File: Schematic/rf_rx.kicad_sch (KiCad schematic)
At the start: 12 parts, among them SW2 TS24CA, U1 ME6217C33M5G, U12 ESP-01F-2M, U13 E28-2G4M27SX

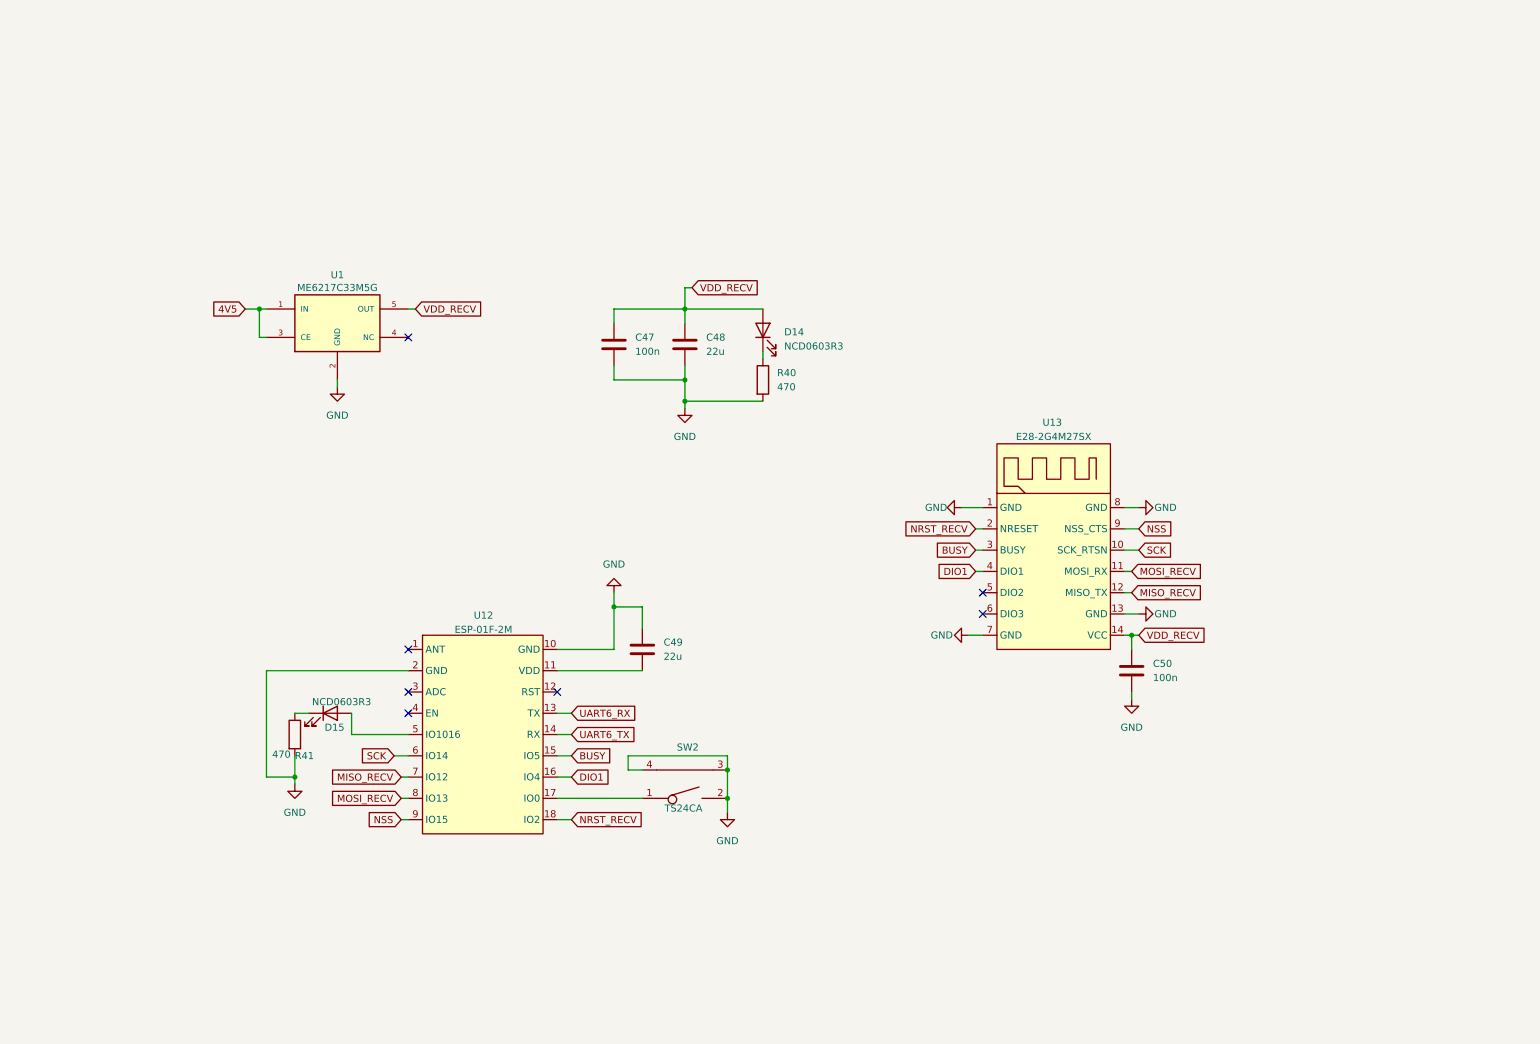
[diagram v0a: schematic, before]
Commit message: Refactor code structure for improved readability and maintainability
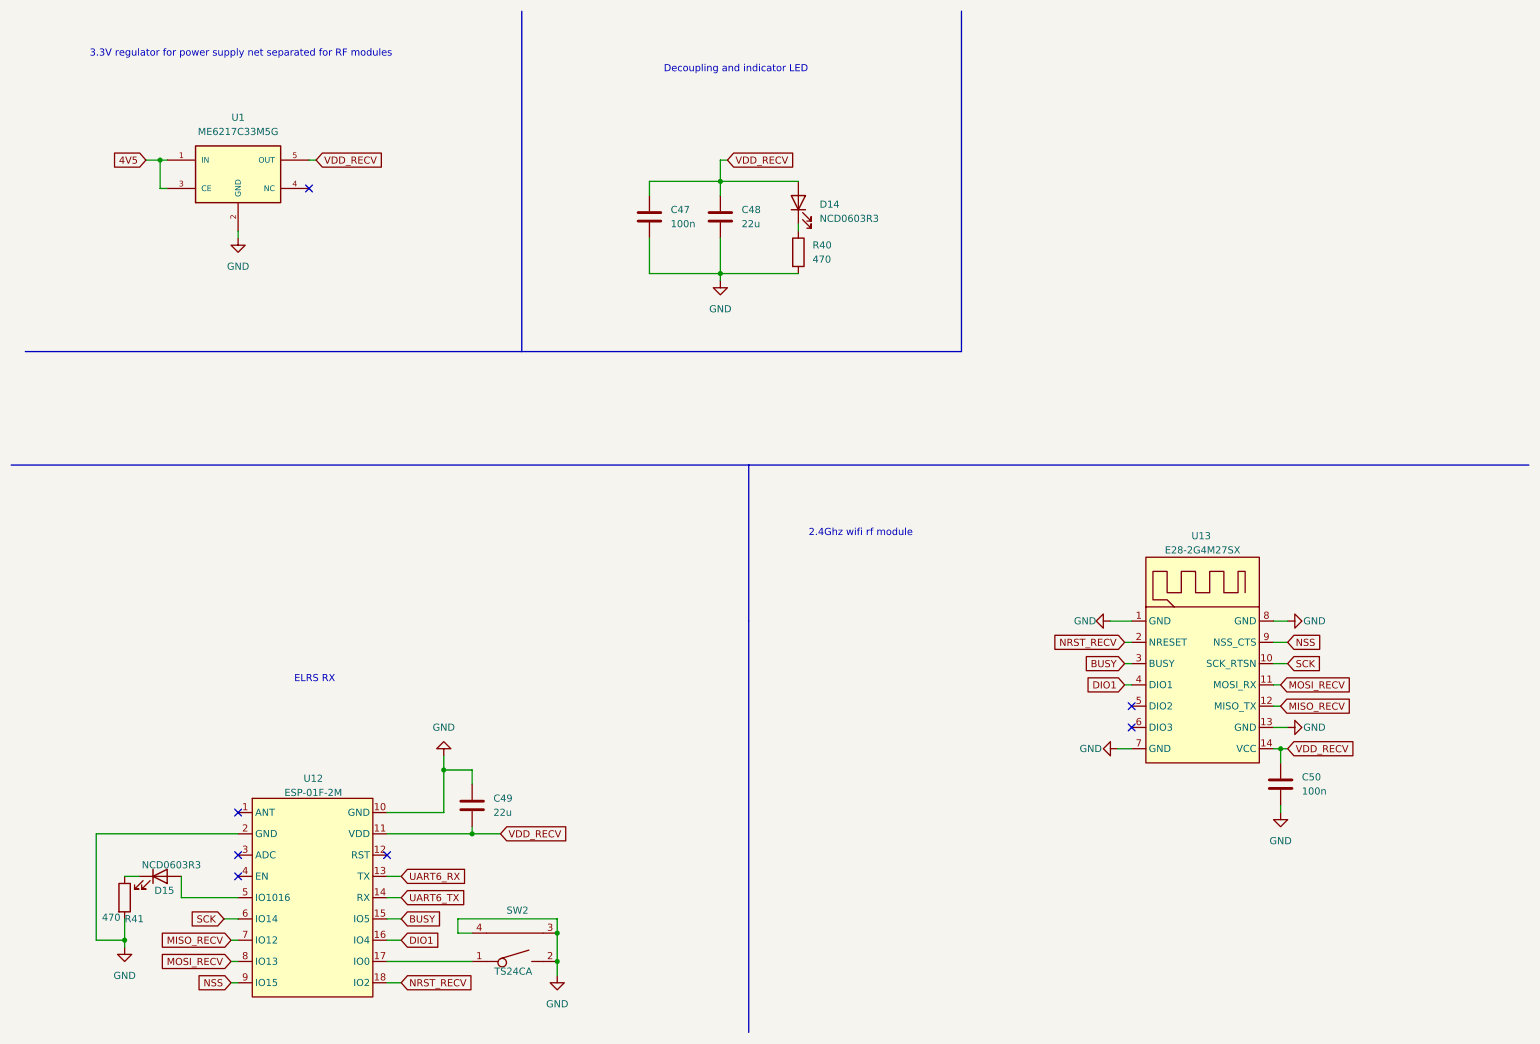
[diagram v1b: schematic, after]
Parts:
- SW2: footprint ProLib_pcs_2025-11-24:SW-SMD_2P-TS24CA -> fch7_fp:SW-SMD_2P-TS24CA
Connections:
- net VDD_RECV: now also C49.2, U12.11 (VDD)
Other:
- note added: "2.4Ghz wifi rf module"
- note added: "3.3V regulator for power supply net separated for RF modules"
- note added: "Decoupling and indicator LED"
- note added: "ELRS RX"
- moved on the sheet: C47, C48, C49, C50, D14, D15, R40, R41, SW2, U1, U12, U13
